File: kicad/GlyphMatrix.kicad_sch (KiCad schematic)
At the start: 36 parts, among them J1 Conn_01x04, SW1 SW_Push, SW2 SW_Push, U1 W25Q128JVS, U2 USBLC6-2SC6, U3 XC6206PxxxMR-Regulator_Linear, Y1 12MHz

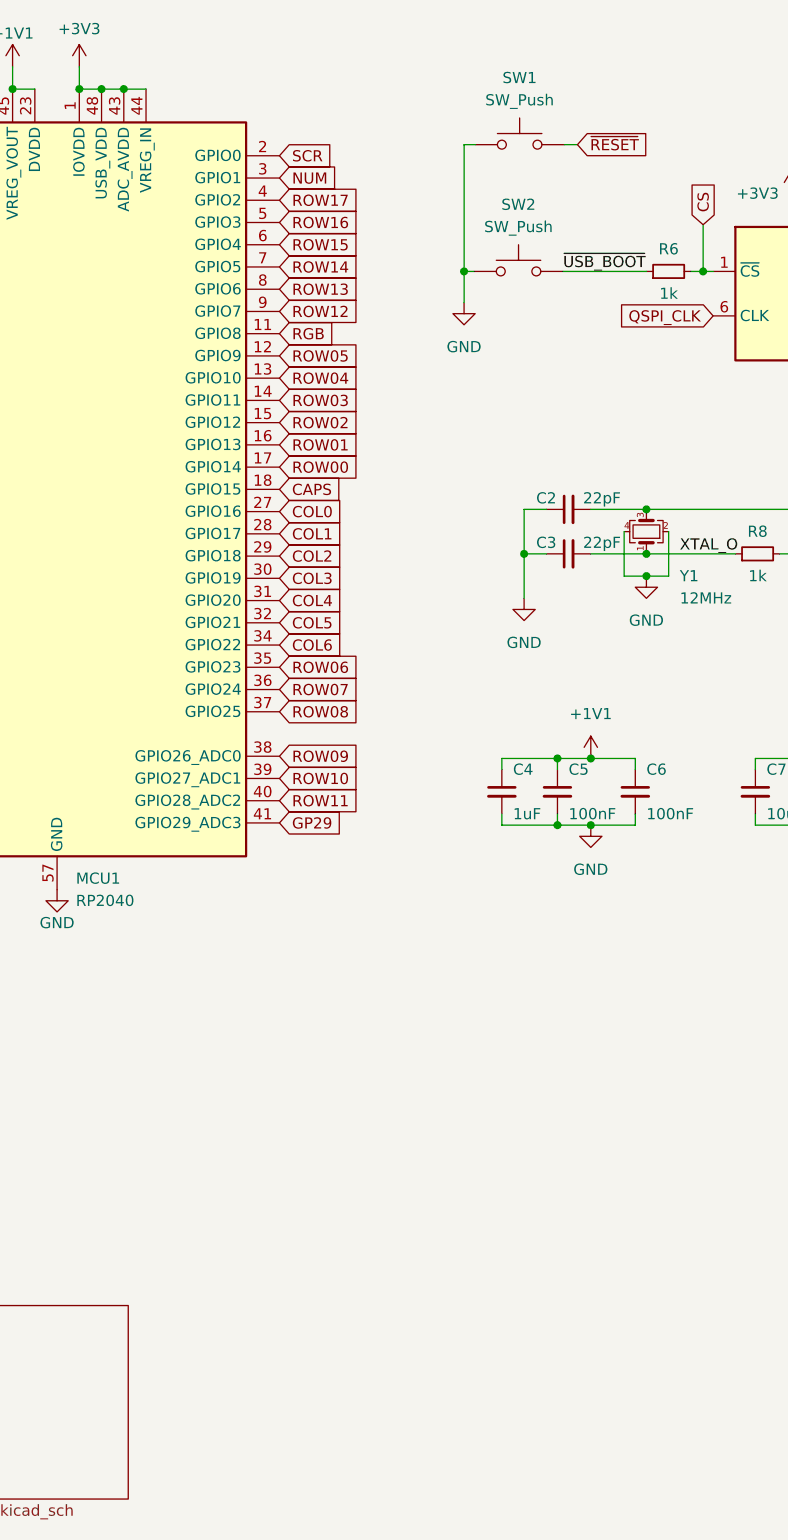
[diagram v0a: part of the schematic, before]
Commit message: artwork
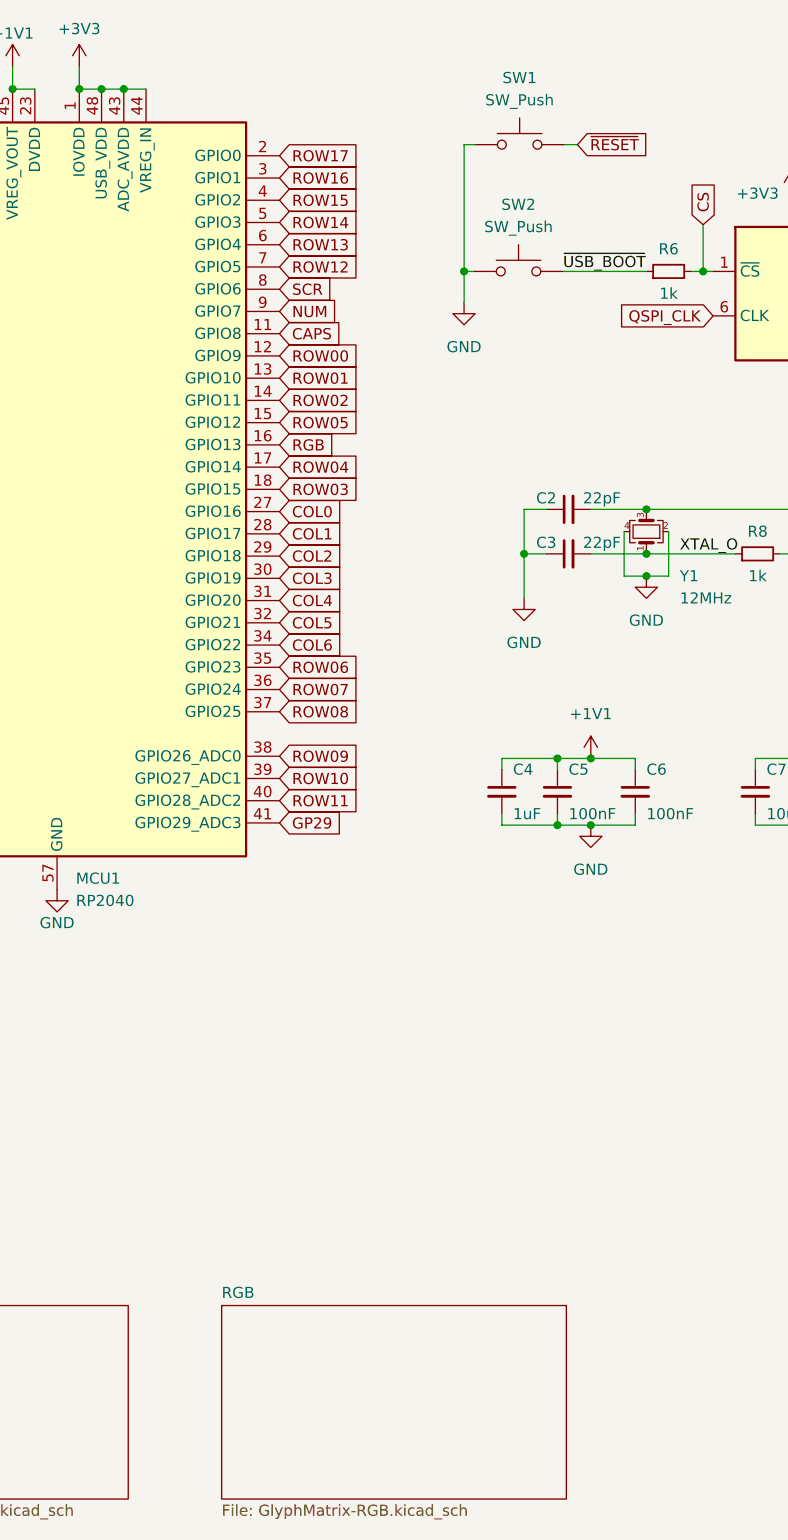
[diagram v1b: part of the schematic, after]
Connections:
- net CAPS: now also MCU1.11 (GPIO8); no longer MCU1.18 (GPIO15)
- net NUM: now also MCU1.9 (GPIO7); no longer MCU1.3 (GPIO1)
- net RGB: now also MCU1.16 (GPIO13); no longer MCU1.11 (GPIO8)
- net ROW00: now also MCU1.12 (GPIO9); no longer MCU1.17 (GPIO14)
- net ROW01: now also MCU1.13 (GPIO10); no longer MCU1.16 (GPIO13)
- net ROW02: now also MCU1.14 (GPIO11); no longer MCU1.15 (GPIO12)
- net ROW03: now also MCU1.18 (GPIO15); no longer MCU1.14 (GPIO11)
- net ROW04: now also MCU1.17 (GPIO14); no longer MCU1.13 (GPIO10)
- net ROW05: now also MCU1.15 (GPIO12); no longer MCU1.12 (GPIO9)
- net ROW12: now also MCU1.7 (GPIO5); no longer MCU1.9 (GPIO7)
- net ROW13: now also MCU1.6 (GPIO4); no longer MCU1.8 (GPIO6)
- net ROW14: now also MCU1.5 (GPIO3); no longer MCU1.7 (GPIO5)
- net ROW15: now also MCU1.4 (GPIO2); no longer MCU1.6 (GPIO4)
- net ROW16: now also MCU1.3 (GPIO1); no longer MCU1.5 (GPIO3)
- net ROW17: now also MCU1.2 (GPIO0); no longer MCU1.4 (GPIO2)
- net SCR: now also MCU1.8 (GPIO6); no longer MCU1.2 (GPIO0)
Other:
- added sheet RGB (GlyphMatrix-RGB.kicad_sch)
- title: (none) -> RP2040 - Keyboard: OmniCode:9001

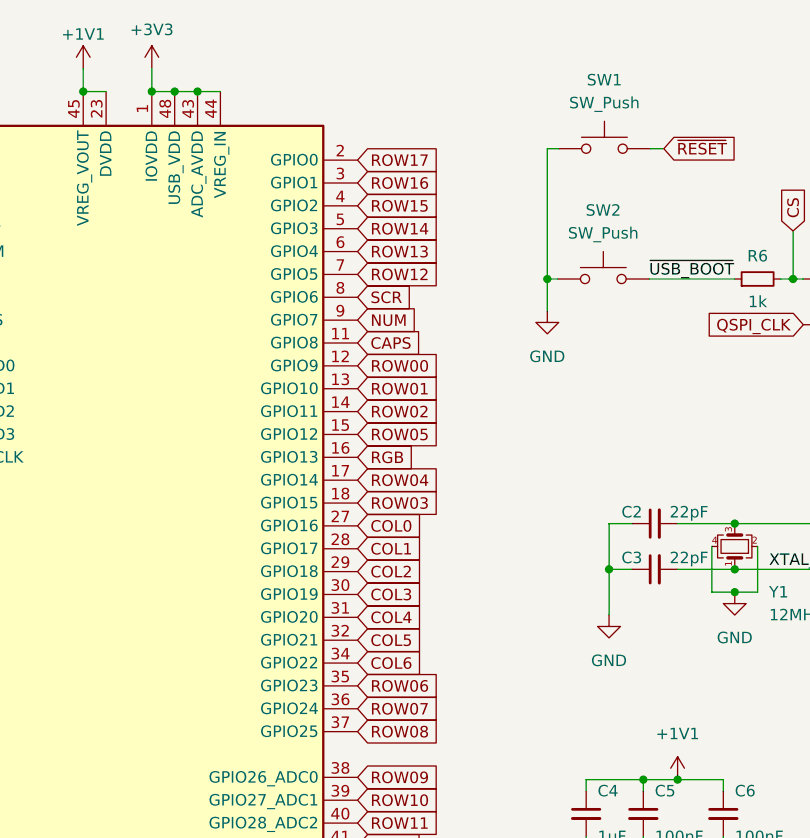
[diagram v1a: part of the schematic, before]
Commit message: artwork #2
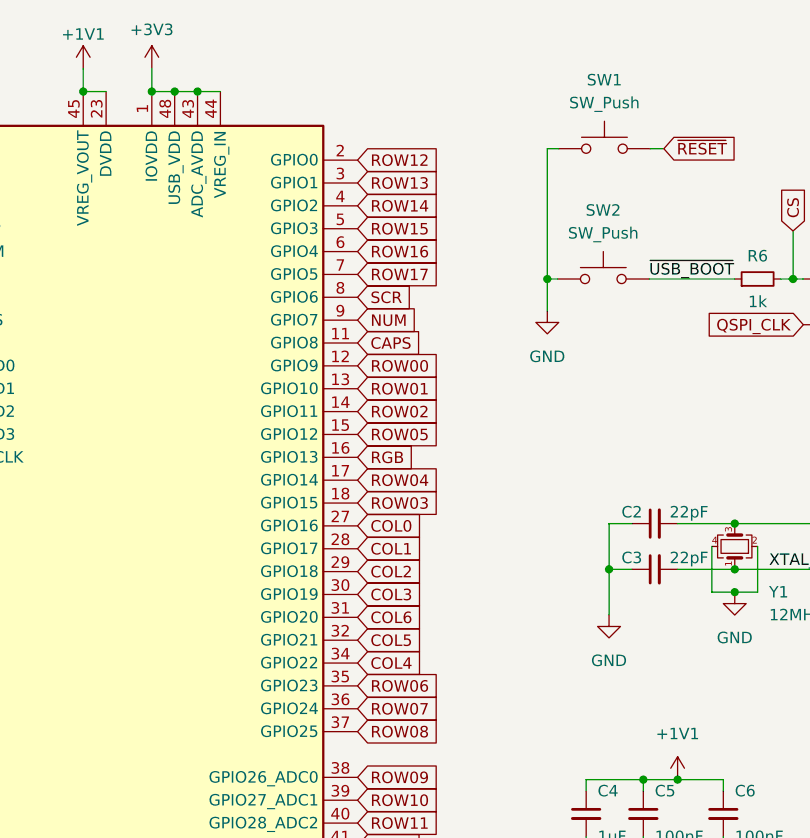
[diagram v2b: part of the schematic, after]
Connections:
- net COL4: now also MCU1.34 (GPIO22); no longer MCU1.31 (GPIO20)
- net COL6: now also MCU1.31 (GPIO20); no longer MCU1.34 (GPIO22)
- net ROW12: now also MCU1.2 (GPIO0); no longer MCU1.7 (GPIO5)
- net ROW13: now also MCU1.3 (GPIO1); no longer MCU1.6 (GPIO4)
- net ROW14: now also MCU1.4 (GPIO2); no longer MCU1.5 (GPIO3)
- net ROW15: now also MCU1.5 (GPIO3); no longer MCU1.4 (GPIO2)
- net ROW16: now also MCU1.6 (GPIO4); no longer MCU1.3 (GPIO1)
- net ROW17: now also MCU1.7 (GPIO5); no longer MCU1.2 (GPIO0)

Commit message: kibot
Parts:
- LED1: LCSC C84264 -> C965808
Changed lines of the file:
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@@
 			)
 		)
-		(property "LCSC" "C84264"
+		(property "LCSC" "C965808"
 			(at 209.55 43.815 0)
 			(effects

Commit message: reorg schematic (#18)
* GlyphMatrix

* PhaseShift

* DeltaForm
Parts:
- removed C1, C10, C11, C12, C13, C14, C15, C5, C6, C9: 100nF, Capacitor_SMD:C_0402_1005Metric, symbol Device:C_Small
- removed C16, C17, C4, C8: 1uF, Capacitor_SMD:C_0402_1005Metric, symbol Device:C_Small
- removed C2, C3: 22pF, Capacitor_SMD:C_0402_1005Metric, symbol Device:C_Small
- removed C7: 10uF, Capacitor_SMD:C_0402_1005Metric, symbol Device:C_Small
- removed F1: 500mA, Fuse:Fuse_1206_3216Metric, symbol Device:Polyfuse_Small
- removed J1: Conn_01x04, Connector_PinHeader_2.00mm:PinHeader_2x02_P2.00mm_Vertical_SMD, symbol Connector_Generic:Conn_01x04
- removed LED1: WHITE, LED_SMD:LED_0603_1608Metric_Pad1.05x0.95mm_HandSolder, symbol Device:LED
- removed MCU1: RP2040, TB2086_SMD_G:RP2040-QFN-56, symbol MCU_RaspberryPi:RP2040
- removed R1, R6, R8: 1k, Resistor_SMD:R_0402_1005Metric, symbol Device:R_Small
- removed R2, R3: 5k1, Resistor_SMD:R_0402_1005Metric, symbol Device:R_Small
- removed R4, R5: 27R, Resistor_SMD:R_0603_1608Metric, symbol Device:R_Small
- removed R7: 330, Resistor_SMD:R_0603_1608Metric, symbol Device:R_Small
- removed SW1, SW2: SW_Push, Button_Switch_SMD:SW_SPST_SKQG_WithoutStem, symbol Switch:SW_Push
- removed U1: W25Q128JVS, Package_SO:SOIC-8_5.3x5.3mm_P1.27mm, symbol Memory_Flash:W25Q128JVS
- removed U2: USBLC6-2SC6, Package_TO_SOT_SMD:SOT-23-6, symbol Power_Protection:USBLC6-2SC6
- removed U3: XC6206PxxxMR-Regulator_Linear, Package_TO_SOT_SMD:SOT-23, symbol kicad-keyboard-parts:XC6206PxxxMR-Regulator_Linear
- removed USB1: USB_C_Receptacle_USB2.0, TB2086_SMD:GCT_USB4520-03-0-A_REVA, symbol Connector:USB_C_Receptacle_USB2.0
- removed Y1: 12MHz, Crystal:Crystal_SMD_3225-4Pin_3.2x2.5mm, symbol Device:Crystal_GND24_Small
- added D1, D10, D11, D12, D13, D14, D15, D16, D17, D18, D19, D2, D20, D21, D22, D23, D24, D25, D26, D27, D28, D29, D3, D30, D31, D32, D33, D34, D35, D36, D37, D38, D39, D4, D40, D41, D42, D43, D44, D45, D46, D47, D48, D49, D5, D50, D51, D52, D53, D54, D55, D56, D57, D58, D59, D6, D60, D61, D62, D63, D64, D65, D66, D67, D68, D69, D7, D70, D71, D72, D73, D74, D8, D9: 1N4148W, TB2086_SMD:D3_SMD, symbol Device:D
- added H1, H2, H3, H4, H5, H6, H7, H8: MountingHole_Pad, TB2086_MISC:MountingHole_2.2mm_M2_Pad, symbol TB2086_MISC:MountingHole_Pad
- added LED2: GREEN, LED_SMD:LED_0603_1608Metric_Pad1.05x0.95mm_HandSolder, symbol Device:LED
- added POGO1, POGO2: Conn_01x05, TB2086_MISC:Pogopin_1x05_P2.54mm_Curved, symbol Connector_Generic:Conn_01x05
- added POGO3, POGO4, POGO5, POGO6: Conn_01x07, TB2086_MISC:Pogopin_1x07_P2.54mm_Curved, symbol Connector_Generic:Conn_01x07
- added R9: 330, Resistor_SMD:R_0603_1608Metric, symbol Device:R_Small
- added S1, S10, S11, S12, S13, S14, S15, S16, S17, S18, S19, S2, S20, S21, S22, S23, S24, S25, S26, S27, S28, S29, S3, S30, S31, S32, S33, S34, S35, S36, S37, S38, S39, S4, S40, S41, S42, S43, S44, S45, S46, S47, S48, S49, S5, S50, S51, S52, S53, S54, S55, S56, S57, S58, S59, S6, S60, S61, S62, S63, S7, S8, S9: SW_MX_HS, TB2086_KEYSWITCH:SW_MX_HS_1u, symbol TB2086_KEYSWITCH:SW_MX_HS
- added S64: SW_MX_HS, TB2086_KEYSWITCH:SW_MX_HS_1.25u, symbol TB2086_KEYSWITCH:SW_MX_HS
- added S65, S66: SW_MX_HS, TB2086_KEYSWITCH:SW_MX_HS_1.5u, symbol TB2086_KEYSWITCH:SW_MX_HS
- added S67, S68, S69: SW_MX_HS, TB2086_KEYSWITCH:SW_MX_HS_1.75u, symbol TB2086_KEYSWITCH:SW_MX_HS
- added S70: SW_MX_HS, TB2086_KEYSWITCH:SW_MX_HS_2u, symbol TB2086_KEYSWITCH:SW_MX_HS
- added S71, S72: SW_MX_HS, TB2086_KEYSWITCH:SW_MX_HS_2.25u, symbol TB2086_KEYSWITCH:SW_MX_HS
- added S73: SW_MX_HS, TB2086_KEYSWITCH:SW_MX_HS_2.75u, symbol TB2086_KEYSWITCH:SW_MX_HS
- added S74: SW_MX_HS, TB2086_KEYSWITCH:SW_MX_HS_6.25u, symbol TB2086_KEYSWITCH:SW_MX_HS
- added STB1, STB2, STB3, STB4: Stabilizer_Cherry_MX_2.00u, Stabilizer_Cherry_MX_2.00u, symbol PCM_marbastlib-mx:MX_stab
- added STB5: Stabilizer_Cherry_MX_6.25u, Stabilizer_Cherry_MX_6.25u, symbol PCM_marbastlib-mx:MX_stab
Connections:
- net +5V: now also POGO1.4 (Pin_4), POGO2.2 (Pin_2)
- net CAPS: now also LED2.2 (A)
- net COL0: now also POGO3.1 (Pin_1), POGO4.7 (Pin_7), S1.2, S13.2, S14.2, S65.2, S66.2, S67.2, S68.2, S69.2, S70.2, S71.2, S72.2, S73.2
- net COL1: now also POGO3.2 (Pin_2), POGO4.6 (Pin_6), S12.2, S15.2, S26.2, S27.2, S38.2, S39.2, S50.2, S60.2
- net COL2: now also POGO3.3 (Pin_3), POGO4.5 (Pin_5), S11.2, S16.2, S2.2, S25.2, S28.2, S37.2, S40.2, S49.2, S51.2, S63.2, S64.2
- net COL3: now also POGO3.4 (Pin_4), POGO4.4 (Pin_4), S10.2, S17.2, S24.2, S29.2, S3.2, S36.2, S41.2, S48.2, S52.2, S59.2, S62.2
- net COL4: now also POGO3.7 (Pin_7), POGO4.1 (Pin_1), S18.2, S23.2, S30.2, S35.2, S4.2, S42.2, S47.2, S53.2, S58.2, S61.2, S9.2
- net COL5: now also POGO3.6 (Pin_6), POGO4.2 (Pin_2), S19.2, S22.2, S31.2, S34.2, S43.2, S46.2, S5.2, S54.2, S57.2, S74.2, S8.2
- net COL6: now also POGO3.5 (Pin_5), POGO4.3 (Pin_3), S20.2, S21.2, S32.2, S33.2, S44.2, S45.2, S55.2, S56.2, S6.2, S7.2
- net GND: now also H1.1, H2.1, H3.1, H4.1, H5.1, H6.1, H7.1, H8.1, POGO1.5 (Pin_5), POGO2.1 (Pin_1), R9.1
- net NUM: now also POGO1.3 (Pin_3), POGO2.3 (Pin_3)
- net ROW00: now also D1.1 (K), D2.1 (K), D3.1 (K), D4.1 (K), D5.1 (K), D6.1 (K)
- net ROW01: now also D14.1 (K), D15.1 (K), D16.1 (K), D17.1 (K), D18.1 (K), D19.1 (K), D20.1 (K)
- net ROW02: now also D27.1 (K), D28.1 (K), D29.1 (K), D30.1 (K), D31.1 (K), D32.1 (K), D65.1 (K)
- net ROW03: now also D39.1 (K), D40.1 (K), D41.1 (K), D42.1 (K), D43.1 (K), D44.1 (K), D67.1 (K)
- net ROW04: now also D50.1 (K), D51.1 (K), D52.1 (K), D53.1 (K), D54.1 (K), D55.1 (K), D72.1 (K)
- net ROW05: now also D60.1 (K), D64.1 (K), D68.1 (K), D74.1 (K)
- net ROW06: now also D10.1 (K), D11.1 (K), D12.1 (K), D13.1 (K), D7.1 (K), D8.1 (K), D9.1 (K)
- net ROW07: now also D21.1 (K), D22.1 (K), D23.1 (K), D24.1 (K), D25.1 (K), D26.1 (K), D70.1 (K)
- net ROW08: now also D33.1 (K), D34.1 (K), D35.1 (K), D36.1 (K), D37.1 (K), D38.1 (K), D66.1 (K)
- net ROW09: now also D45.1 (K), D46.1 (K), D47.1 (K), D48.1 (K), D49.1 (K), D71.1 (K)
- net ROW10: now also D56.1 (K), D57.1 (K), D58.1 (K), D59.1 (K), D73.1 (K)
- net ROW11: now also D61.1 (K), D62.1 (K), D63.1 (K), D69.1 (K)
- net ROW12: now also POGO5.1 (Pin_1), POGO6.7 (Pin_7)
- net ROW13: now also POGO5.2 (Pin_2), POGO6.6 (Pin_6)
- net ROW14: now also POGO5.3 (Pin_3), POGO6.5 (Pin_5)
- net ROW15: now also POGO5.4 (Pin_4), POGO6.4 (Pin_4)
- net ROW16: now also POGO5.5 (Pin_5), POGO6.3 (Pin_3)
- net ROW17: now also POGO5.6 (Pin_6), POGO6.2 (Pin_2)
- net SCR: now also POGO1.2 (Pin_2), POGO2.4 (Pin_4)
- new net: D23.2 (A), S23.1
- new net: D21.2 (A), S21.1
- new net: D34.2 (A), S34.1
- new net: D30.2 (A), S30.1
- new net: D11.2 (A), S11.1
- new net: D27.2 (A), S27.1
- new net: D2.2 (A), S2.1
- new net: D63.2 (A), S63.1
- new net: D71.2 (A), S71.1
- new net: D16.2 (A), S16.1
- new net: D66.2 (A), S66.1
- new net: D41.2 (A), S41.1
- new net: D39.2 (A), S39.1
- new net: D69.2 (A), S69.1
- new net: D19.2 (A), S19.1
- new net: D32.2 (A), S32.1
- new net: D46.2 (A), S46.1
- new net: D53.2 (A), S53.1
- new net: D54.2 (A), S54.1
- new net: D26.2 (A), S26.1
- new net: D59.2 (A), S59.1
- new net: D14.2 (A), S14.1
- new net: D9.2 (A), S9.1
- new net: D15.2 (A), S15.1
- new net: D67.2 (A), S67.1
- new net: D64.2 (A), S64.1
- new net: D73.2 (A), S73.1
- new net: D60.2 (A), S60.1
- new net: D50.2 (A), S50.1
- new net: D44.2 (A), S44.1
- new net: D37.2 (A), S37.1
- new net: D25.2 (A), S25.1
- new net: D72.2 (A), S72.1
- new net: D40.2 (A), S40.1
- new net: D70.2 (A), S70.1
- new net: D20.2 (A), S20.1
- new net: D45.2 (A), S45.1
- new net: D57.2 (A), S57.1
- new net: LED2.1 (K), R9.2
- new net: D74.2 (A), S74.1
- new net: D55.2 (A), S55.1
- new net: D10.2 (A), S10.1
- new net: D43.2 (A), S43.1
- new net: D28.2 (A), S28.1
- new net: D31.2 (A), S31.1
- new net: D29.2 (A), S29.1
- new net: D22.2 (A), S22.1
- new net: D52.2 (A), S52.1
- new net: D68.2 (A), S68.1
- new net: D56.2 (A), S56.1
- new net: D61.2 (A), S61.1
- new net: D4.2 (A), S4.1
- new net: D38.2 (A), S38.1
- new net: D58.2 (A), S58.1
- new net: D13.2 (A), S13.1
- new net: D36.2 (A), S36.1
- new net: D12.2 (A), S12.1
- new net: D49.2 (A), S49.1
- new net: D33.2 (A), S33.1
- new net: D6.2 (A), S6.1
- new net: D51.2 (A), S51.1
- new net: D3.2 (A), S3.1
- new net: D42.2 (A), S42.1
- new net: D7.2 (A), S7.1
- new net: D18.2 (A), S18.1
- new net: D5.2 (A), S5.1
- new net: D35.2 (A), S35.1
- new net: D47.2 (A), S47.1
- new net: D65.2 (A), S65.1
- new net: D48.2 (A), S48.1
- new net: D24.2 (A), S24.1
- new net: D8.2 (A), S8.1
- new net: D62.2 (A), S62.1
- new net: D17.2 (A), S17.1
- new net: D1.2 (A), S1.1
- new net RGB_FOM_LEFT: POGO1.1 (Pin_1)
- new net RGB_FOM_RIGHT: POGO6.1 (Pin_1)
- new net RGB_TO_LEFT: POGO5.7 (Pin_7)
- new net RGB_TO_RIGHT: POGO2.5 (Pin_5)
- no-connect marks 2 -> 0
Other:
- removed sheet GlyphMatrix
- added sheet RP2040 (GlyphMatrix-RP2040.kicad_sch)
